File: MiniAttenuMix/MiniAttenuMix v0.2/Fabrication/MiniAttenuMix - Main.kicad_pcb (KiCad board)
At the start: 2 copper layers, 50 x 128.5 mm, 55 parts, among them J1 IDC_2x05, U1 TL072, U2 TL072, U3 TL074

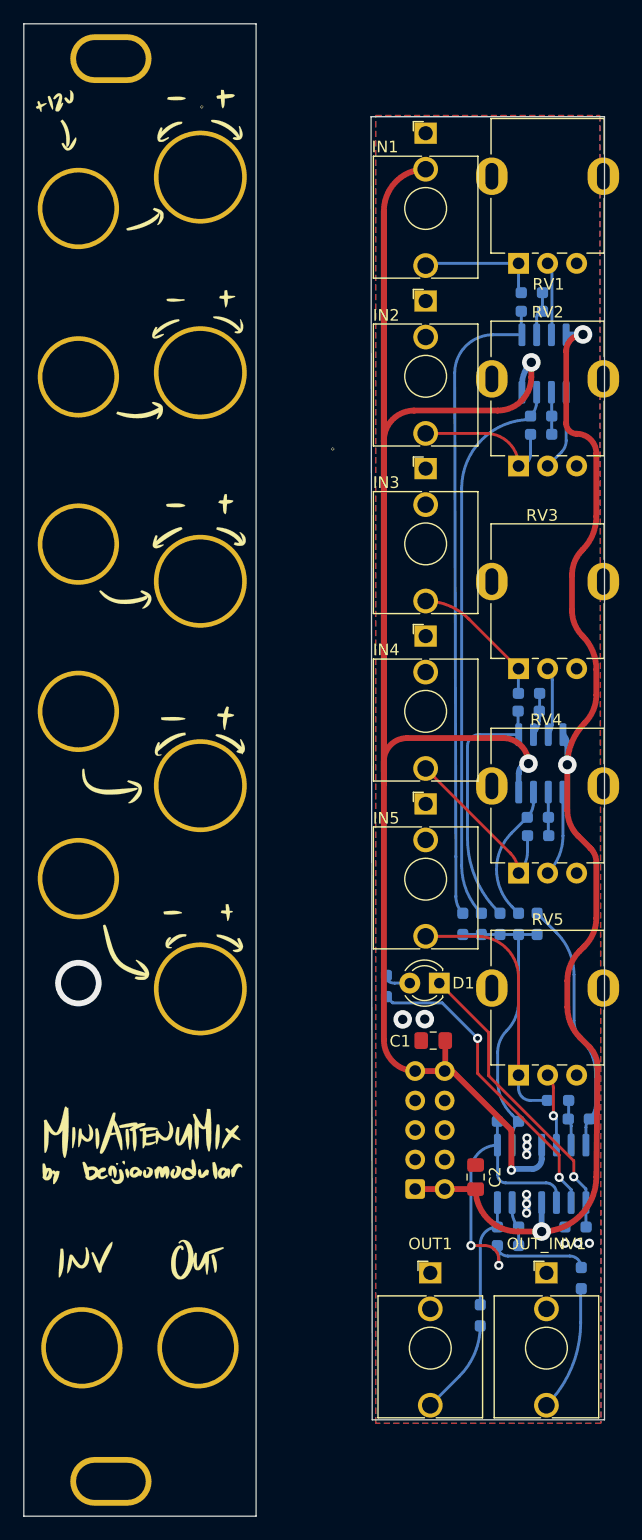
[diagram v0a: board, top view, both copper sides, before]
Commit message: Added v0.2 gerbers
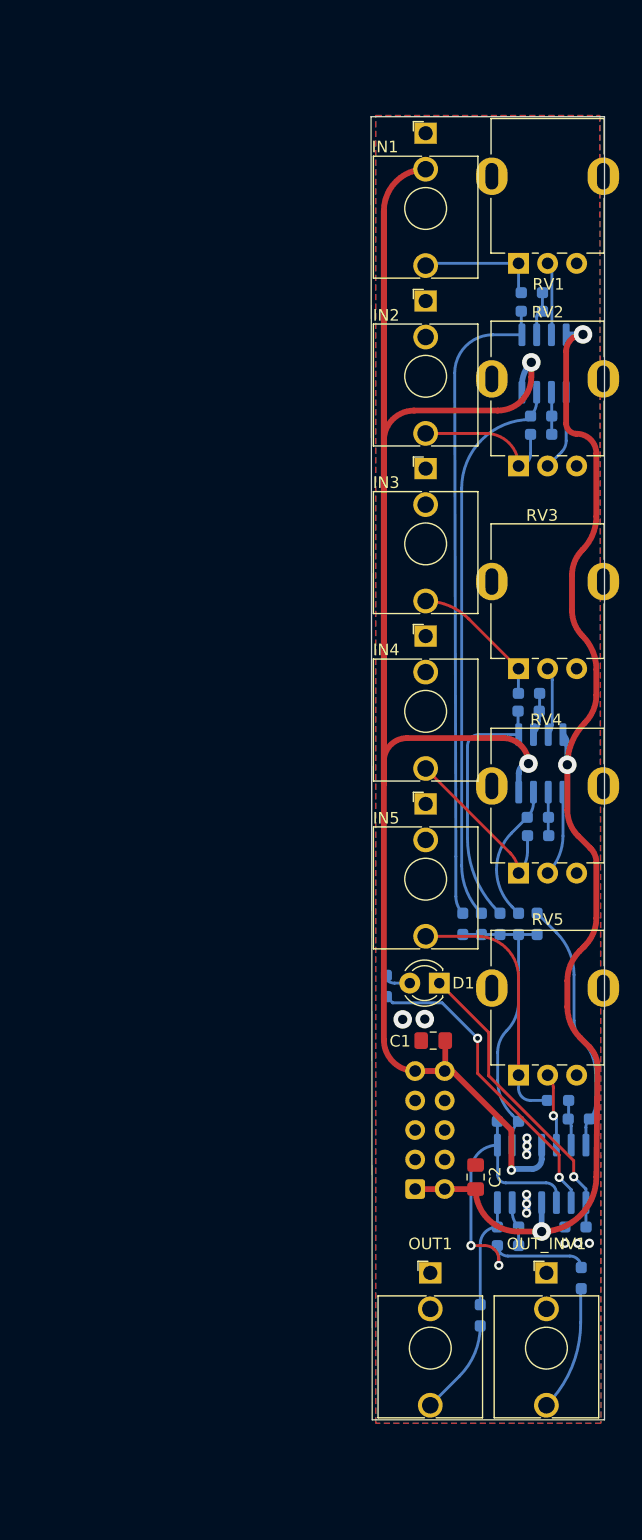
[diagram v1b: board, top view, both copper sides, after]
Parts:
- removed G***: LOGO, LOGO
- removed REF** (x7): PanelHole_AudioJack_3.5mm, benjiaomodular:PanelHole_AudioJack_3.5mm
- removed REF** (x5): PanelHole_Potentiometer_RV09, benjiaomodular:PanelHole_Potentiometer_RV09
- removed REF**: Panel_4HP, benjiaomodular:Panel_4HP
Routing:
- net (no net): vias 1 -> 0
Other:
- board size 50 x 128.5 mm -> 20.1 x 112.2 mm
